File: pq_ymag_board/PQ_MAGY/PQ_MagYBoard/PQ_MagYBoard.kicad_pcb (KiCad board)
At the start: 6 copper layers, 45 x 45 mm, 10 parts, among them J1 M20-7810245

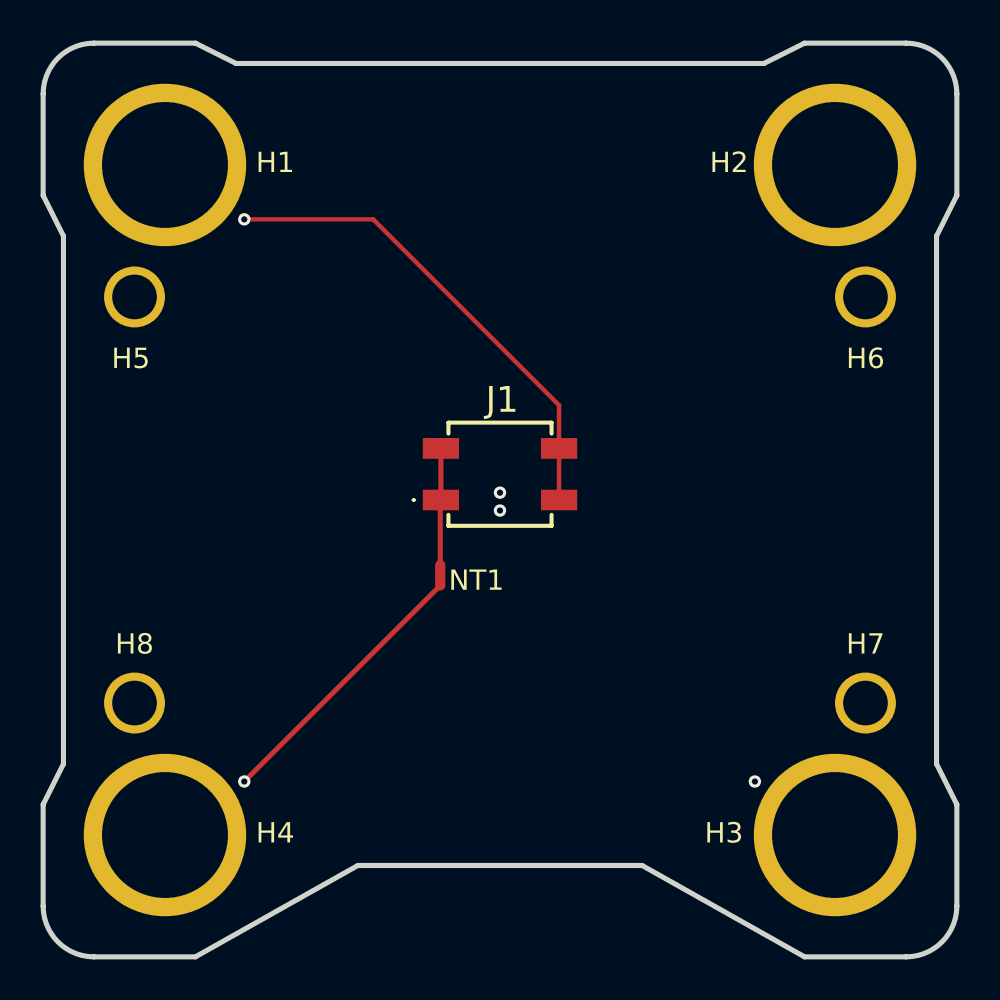
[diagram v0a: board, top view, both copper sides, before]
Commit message: Functional revision and finishing touches part II
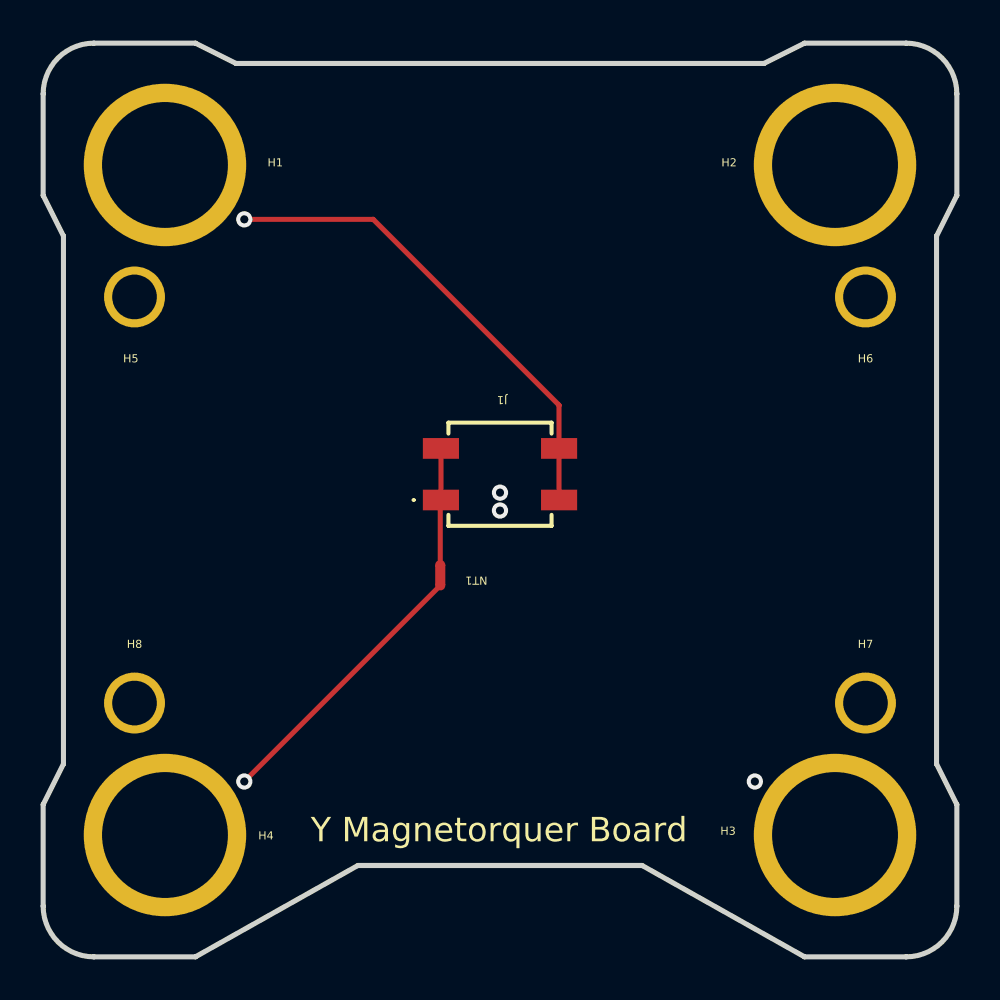
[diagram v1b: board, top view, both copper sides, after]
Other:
- board text added: "Y Magnetorquer Board"
